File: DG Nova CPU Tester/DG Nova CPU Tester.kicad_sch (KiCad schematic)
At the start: 125 parts, among them J1 Slot_02x50_Odd_Even, J10 Programmed I/O, J11 CPU Option Inputs, J12 Data Channel, J13 Program Interrupt, J14 System Control, J17 CPU Option Outputs, J18 MEM Control Outputs, J19 Logic 8 CH, J20 Logic 8 CH, J21 Arduino Anolog Pins, J22 Arduino Digital Pins, J23 Arduino Digital Pins, J4 ATX Power Port, J6 MBO, J7 MEM, J8 Data Channel, J9 Front Panel Controls, SW1 Arduino Mega Reset, SW1 Pico Reset, SW2 Power Swtich, SW4 SW_DIP_x04, U1 74HC14, U2 Pico, U3 74LS08, U4 74LS08

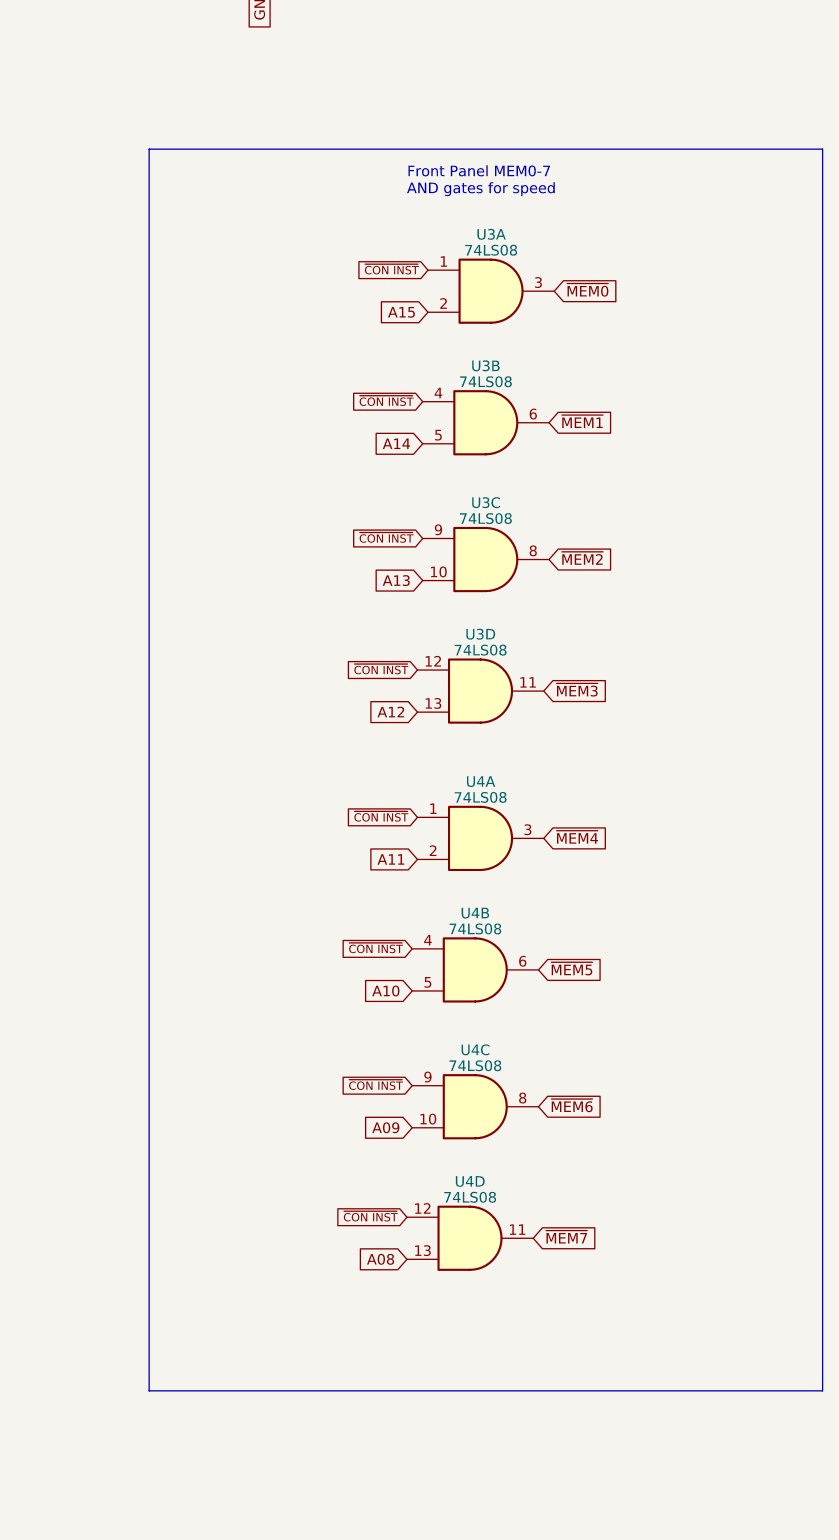
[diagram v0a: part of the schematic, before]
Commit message: Lots o updates
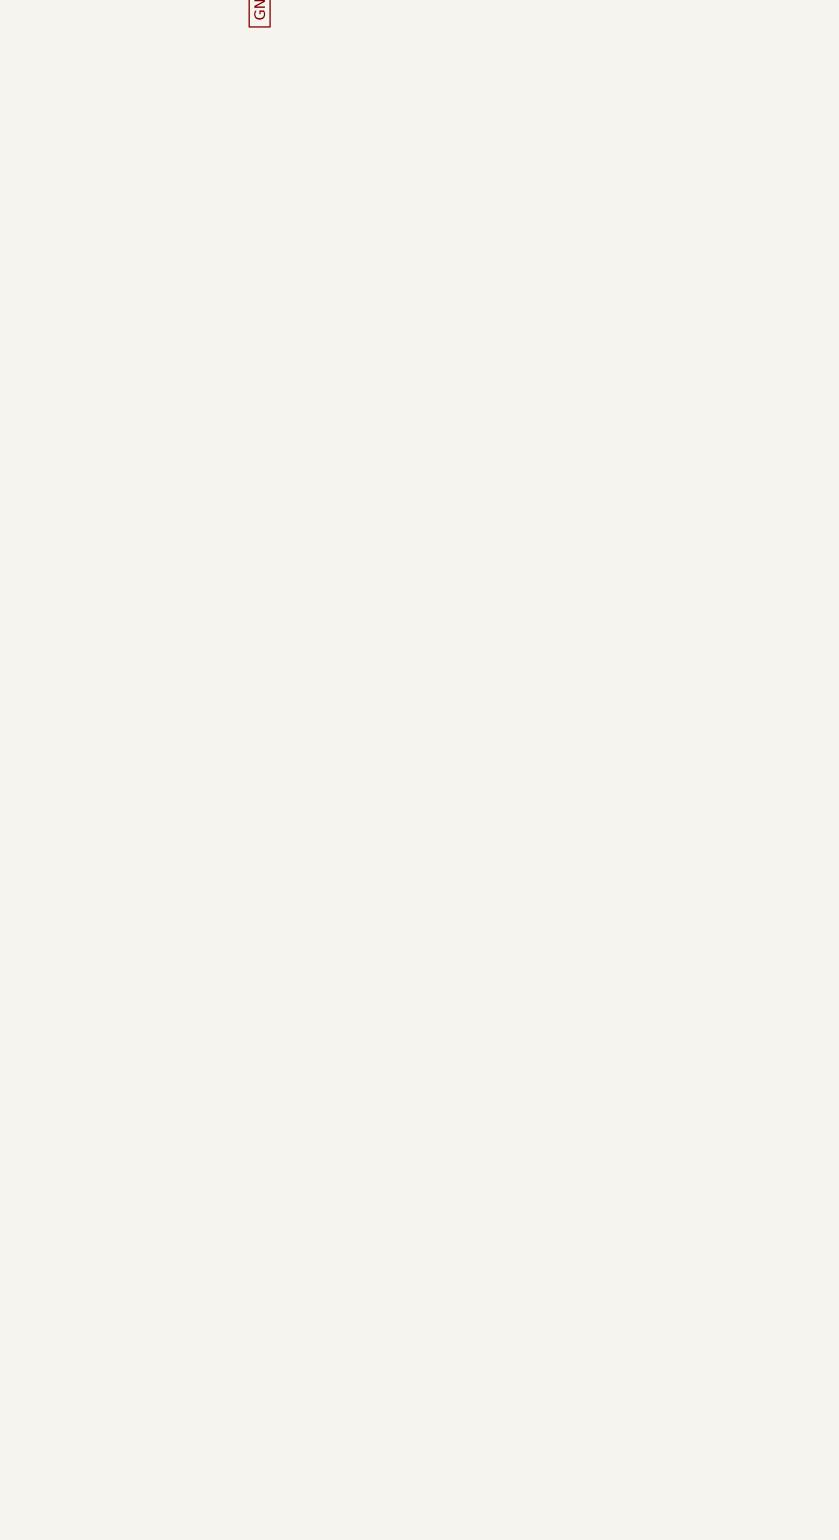
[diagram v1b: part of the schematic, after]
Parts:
- removed unit 2 of U3
- removed unit 1 of U3
- removed unit 3 of U3
- removed unit 4 of U3
- removed unit 4 of U4
- removed unit 3 of U4
- removed unit 2 of U4
- removed unit 1 of U4
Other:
- note removed: "Front Panel MEM0-7 AND gates for speed"
